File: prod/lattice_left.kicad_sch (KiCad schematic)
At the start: 83 parts, among them J1 USB_C_Receptacle, J2 USB_C_Receptacle, SW1 SW_Push, SW2 SW_Push, U1 RP2040, U2 XC6206PxxxMR, U3 USBLC6-2SC6, U4 W25Q128JVS, Y1 12MHz

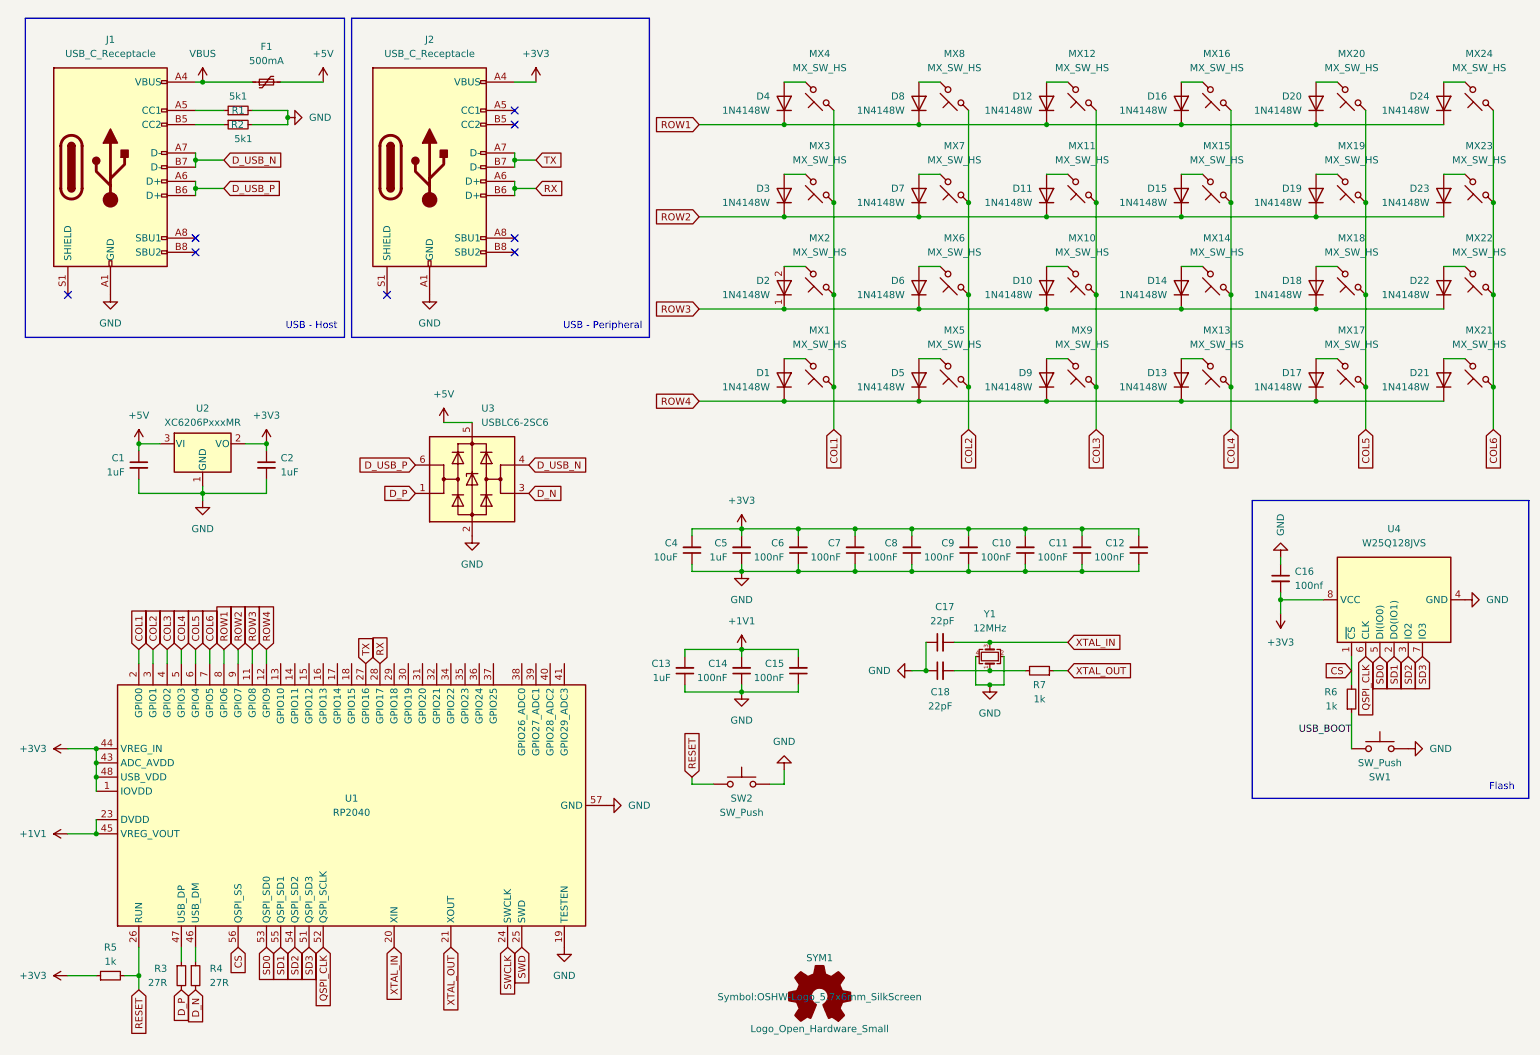
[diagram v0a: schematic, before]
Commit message: components placed
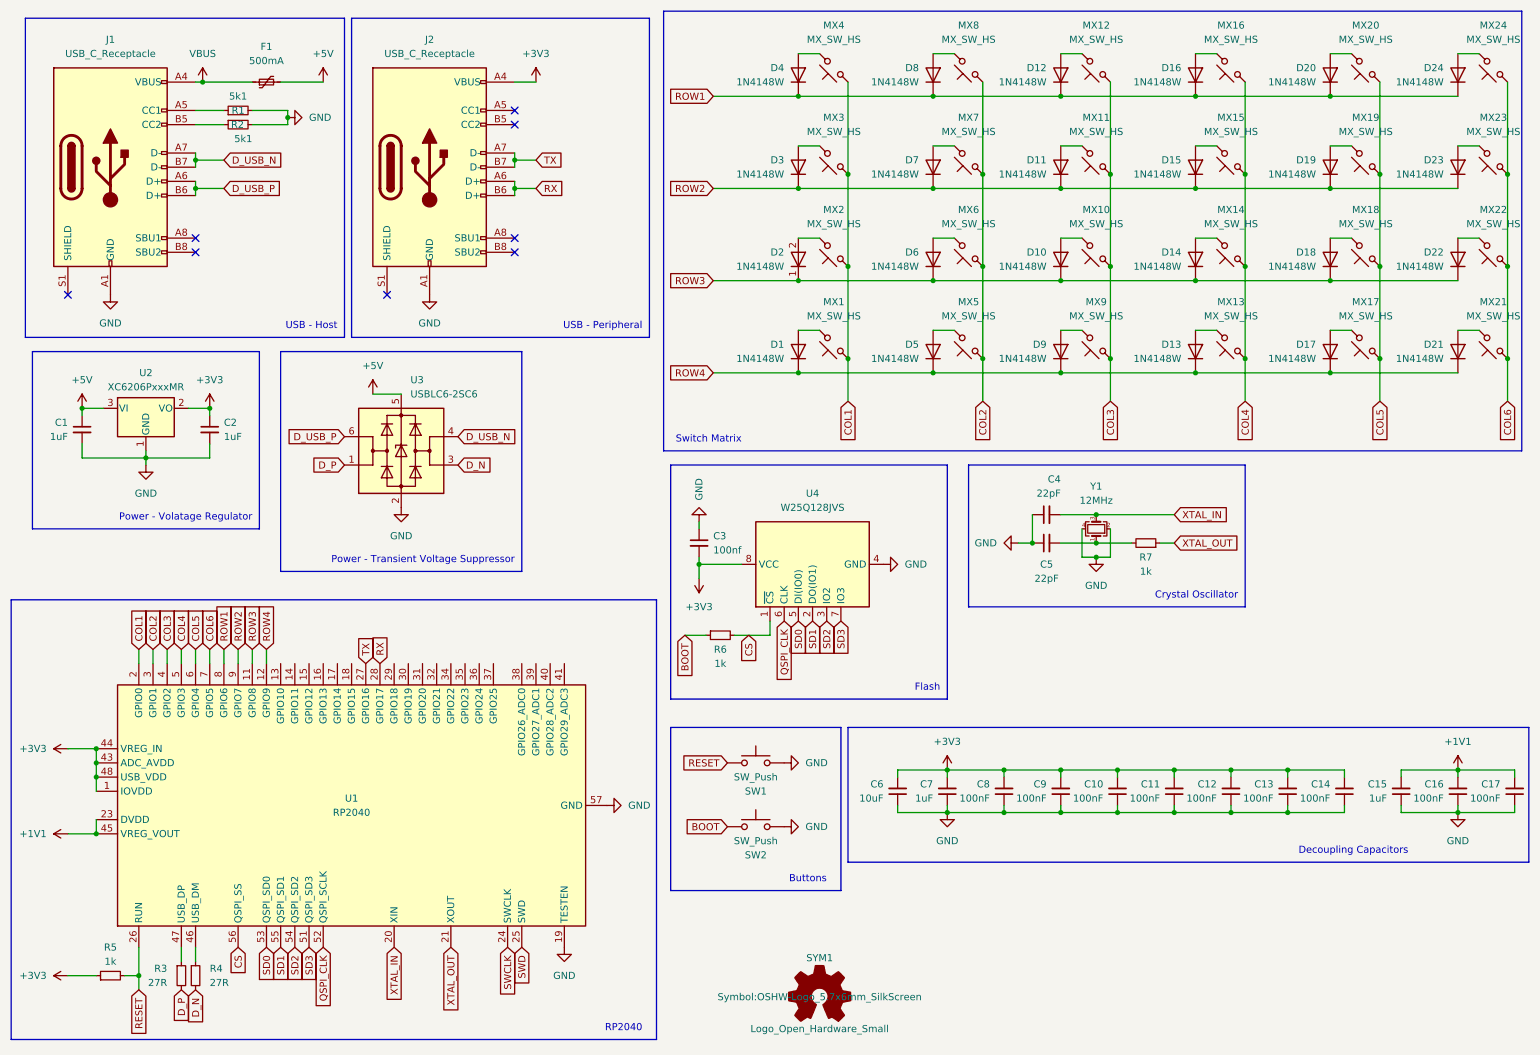
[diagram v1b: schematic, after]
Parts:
- removed SW2: SW_Push, Button_Switch_SMD:SW_SPST_SKQG_WithStem, symbol Switch:SW_Push
- added SW1: SW_Push, Button_Switch_SMD:SW_SPST_SKQG_WithStem, symbol Switch:SW_Push
- renumbered C8 to C10, C9 to C11, C10 to C12, C11 to C13, C12 to C14, C13 to C15, C14 to C16, C15 to C17, C16 to C3, C17 to C4, C18 to C5, C4 to C6, C5 to C7, C6 to C8, C7 to C9, SW1 to SW2
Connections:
- net GND: now also SW1.1
- net RESET: now also SW1.2
- net USB_BOOT renamed BOOT
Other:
- note added: "Buttons"
- note added: "Crystal Oscillator"
- note added: "Decoupling Capacitors"
- note added: "Power - Transient Voltage Suppressor"
- note added: "Power - Volatage Regulator"
- note added: "RP2040"
- note added: "Switch Matrix"
- moved on the sheet: C1, C10, C11, C12, C13, C14, C15, C16, C17, C2, C3, C4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
